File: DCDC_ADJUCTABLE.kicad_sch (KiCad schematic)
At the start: 43 parts, among them Q1001 NVTFWS4D9N04XMTAG, Q1002 NVTFWS4D9N04XMTAG, Q1003 BSS138L, U1001 TPS62933, U1002 LM74700, U1003 TPS62933, U1004 LM74700

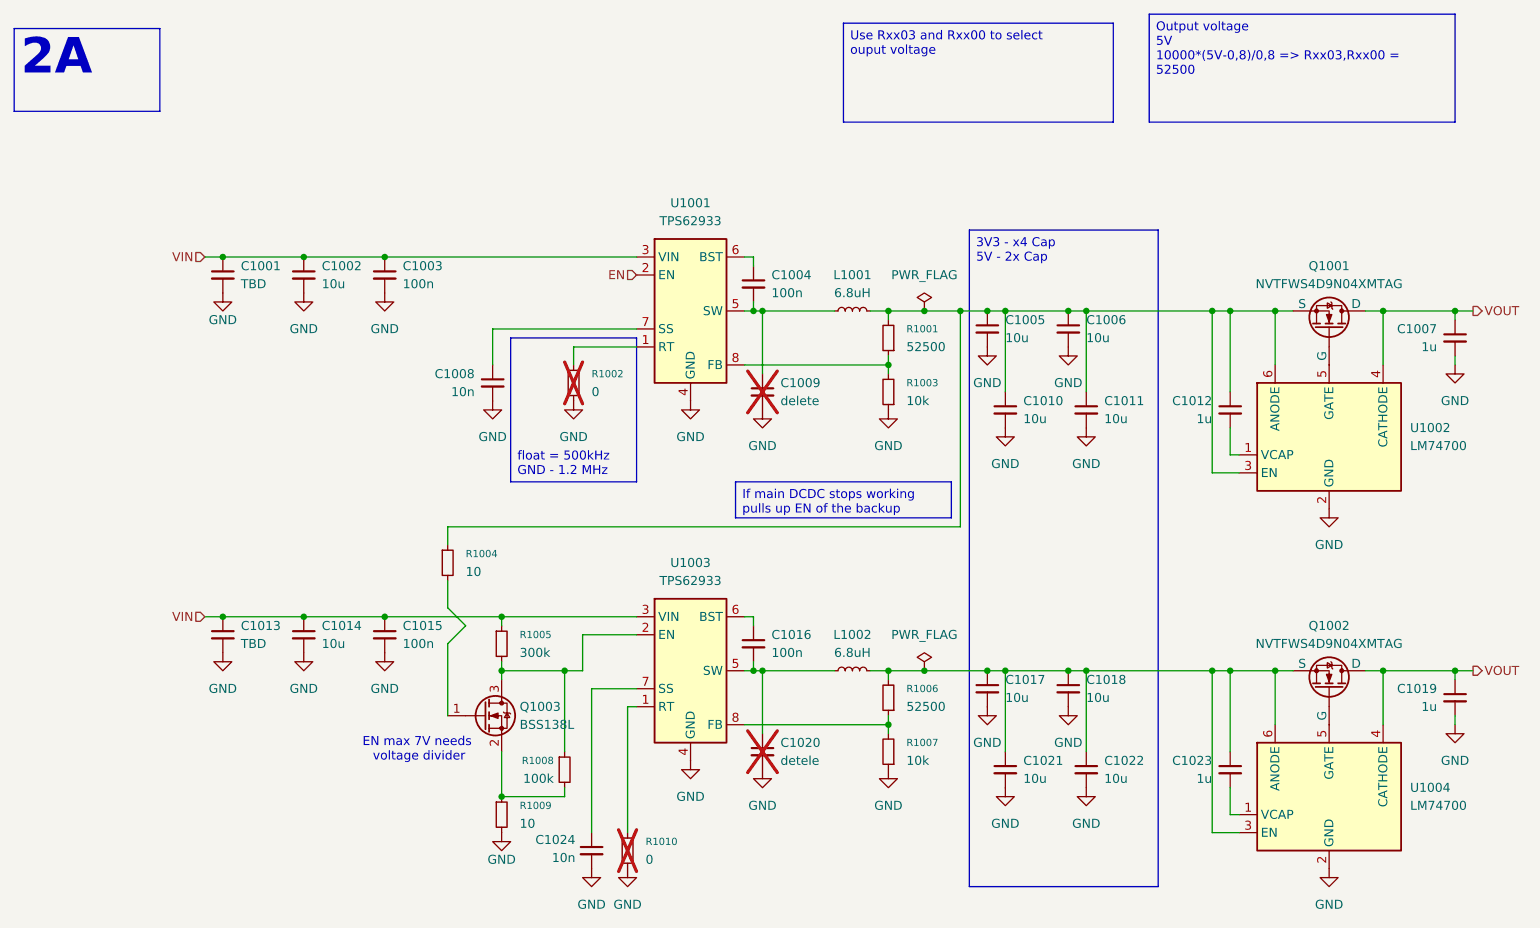
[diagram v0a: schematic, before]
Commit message: small changes to test board
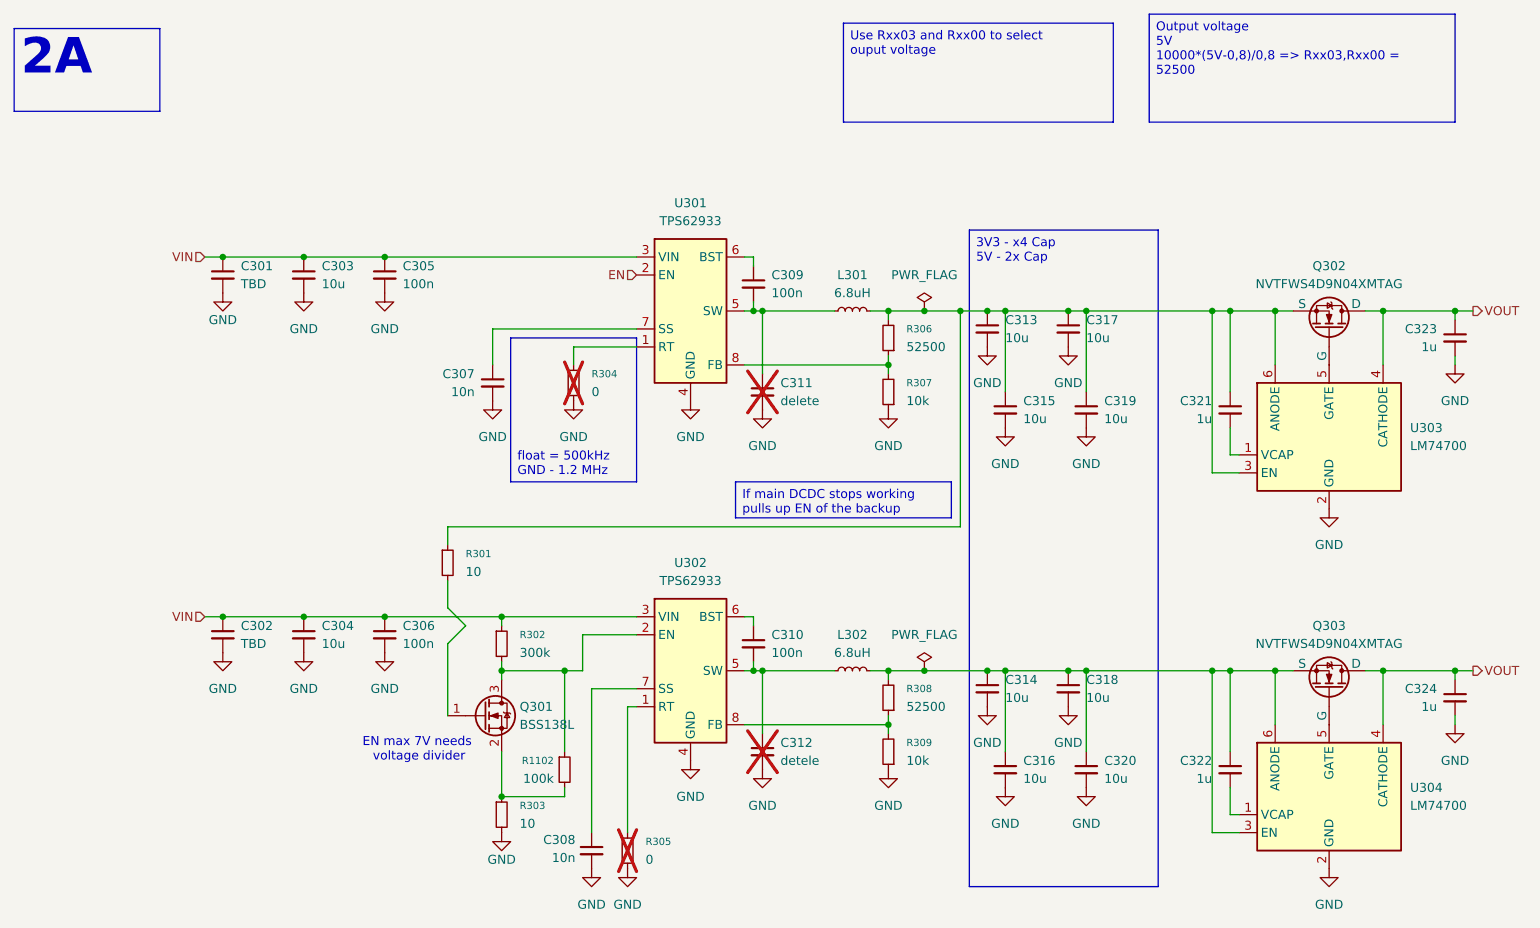
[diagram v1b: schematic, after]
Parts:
- renumbered C1001 to C301, C1013 to C302, C1002 to C303, C1014 to C304, C1003 to C305, C1015 to C306, C1008 to C307, C1024 to C308, C1004 to C309, C1016 to C310, C1009 to C311, C1020 to C312, C1005 to C313, C1017 to C314, C1010 to C315, C1021 to C316, C1006 to C317, C1018 to C318, C1011 to C319, C1022 to C320, C1012 to C321, C1023 to C322, C1007 to C323, C1019 to C324, L1001 to L301, L1002 to L302, Q1003 to Q301, Q1001 to Q302, Q1002 to Q303, R1008 to R1102, R1004 to R301, R1005 to R302, R1009 to R303, R1002 to R304, R1010 to R305, R1001 to R306, R1003 to R307, R1006 to R308, R1007 to R309, U1001 to U301, U1003 to U302, U1002 to U303, U1004 to U304

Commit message: nearly finnished CORE pcb
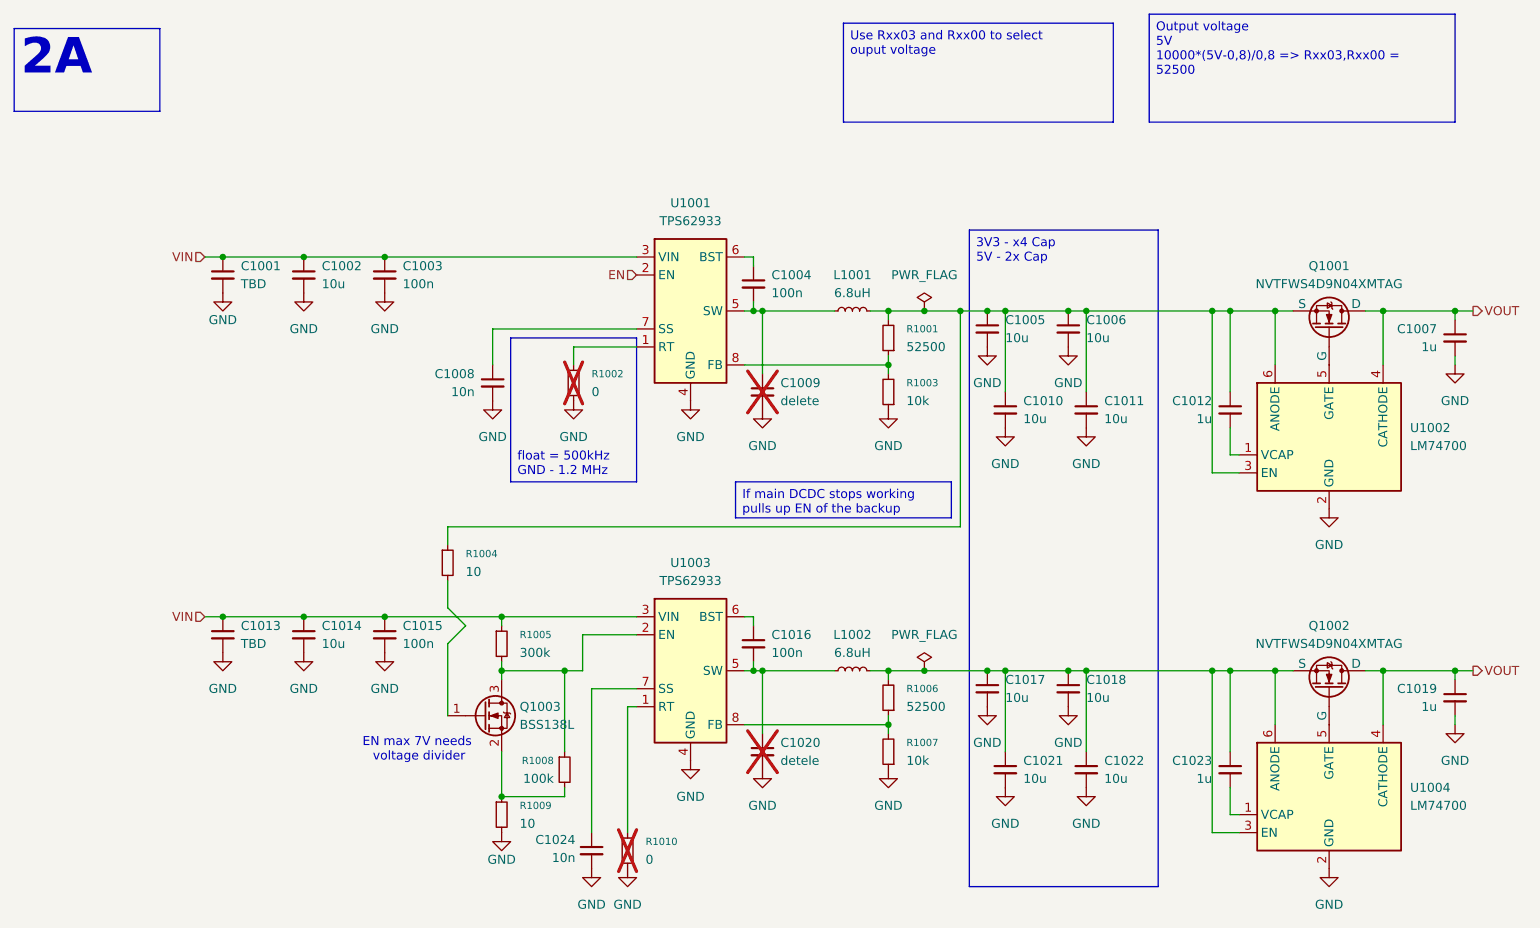
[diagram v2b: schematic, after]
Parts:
- renumbered C301 to C1001, C303 to C1002, C305 to C1003, C309 to C1004, C313 to C1005, C317 to C1006, C323 to C1007, C307 to C1008, C311 to C1009, C315 to C1010, C319 to C1011, C321 to C1012, C302 to C1013, C304 to C1014, C306 to C1015, C310 to C1016, C314 to C1017, C318 to C1018, C324 to C1019, C312 to C1020, C316 to C1021, C320 to C1022, C322 to C1023, C308 to C1024, L301 to L1001, L302 to L1002, Q302 to Q1001, Q303 to Q1002, Q301 to Q1003, R306 to R1001, R304 to R1002, R307 to R1003, R301 to R1004, R302 to R1005, R308 to R1006, R309 to R1007, R1102 to R1008, R303 to R1009, R305 to R1010, U301 to U1001, U303 to U1002, U302 to U1003, U304 to U1004
